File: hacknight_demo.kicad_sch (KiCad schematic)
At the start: 1 part

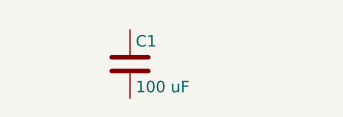
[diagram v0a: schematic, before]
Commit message: tr
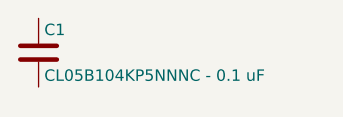
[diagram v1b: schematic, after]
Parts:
- C1: value 100 uF -> CL05B104KP5NNNC - 0.1 uF
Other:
- moved on the sheet: C1
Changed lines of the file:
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@@
 	(symbol
 		(lib_id "Device:C")
-		(at 153.67 88.9 0)
+		(at 143.51 87.63 0)
 		(unit 1)
 		(exclude_from_sim no)
@@
 		(dnp no)
 		(property "Reference" "C1"
-			(at 154.305 86.36 0)
+			(at 144.145 85.09 0)
 			(effects
 				(font
@@
 			)
 		)
-		(property "Value" "100 uF"
-			(at 154.305 91.44 0)
+		(property "Value" "CL05B104KP5NNNC - 0.1 uF"
+			(at 144.145 90.17 0)
 			(effects
 				(font
@@
 		)
 		(property "Footprint" ""
-			(at 154.6352 92.71 0)
+			(at 144.4752 91.44 0)
 			(effects
 				(font
@@
 		)
 		(property "Datasheet" "~"
-			(at 153.67 88.9 0)
+			(at 143.51 87.63 0)
 			(effects
 				(font
@@
 		)
 		(property "Description" "Unpolarized capacitor"
-			(at 153.67 88.9 0)
+			(at 143.51 87.63 0)
 			(effects
 				(font
